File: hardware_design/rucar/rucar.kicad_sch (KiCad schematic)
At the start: 6 parts

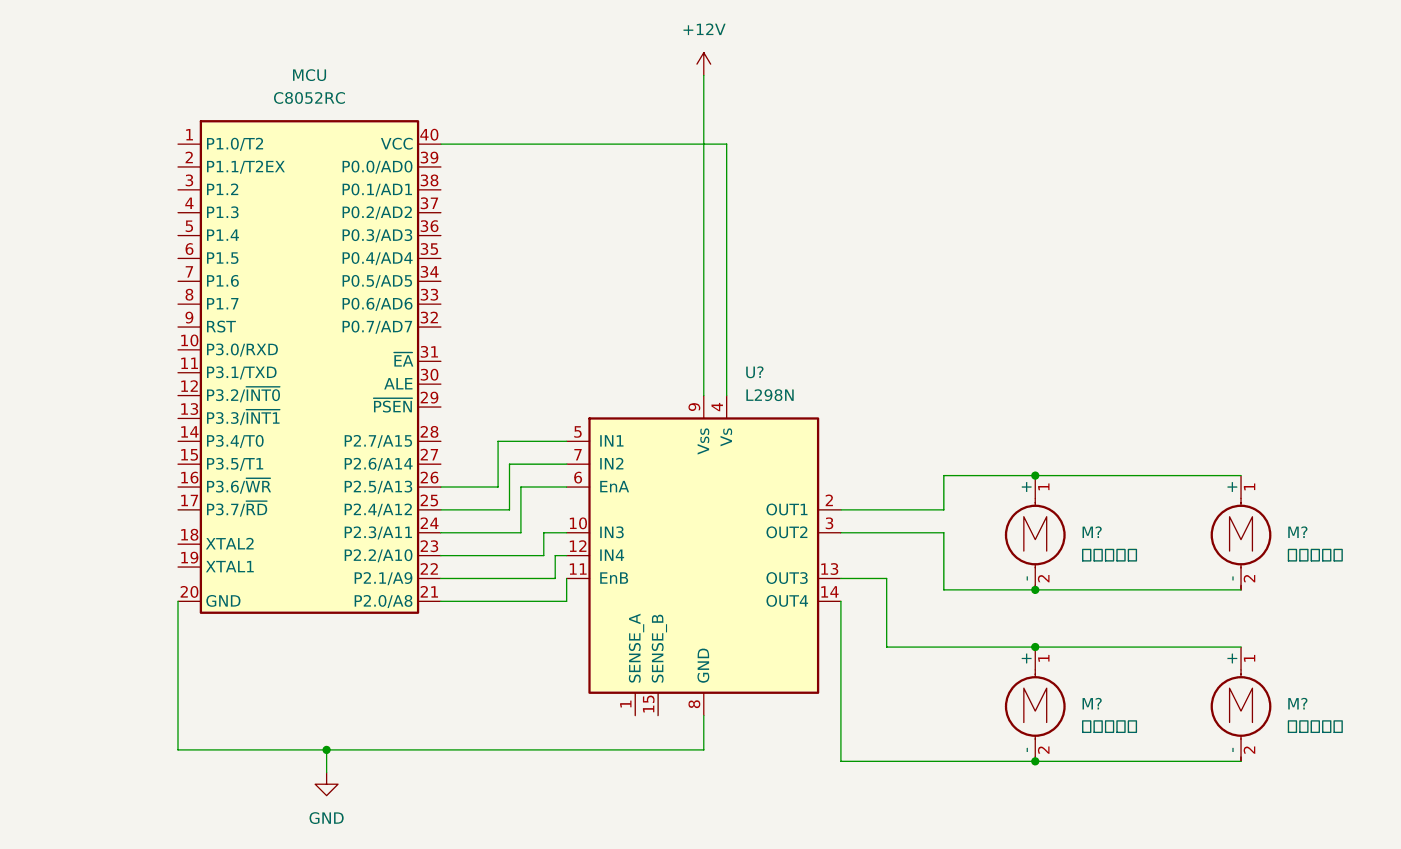
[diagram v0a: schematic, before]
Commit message: finish hardware design.
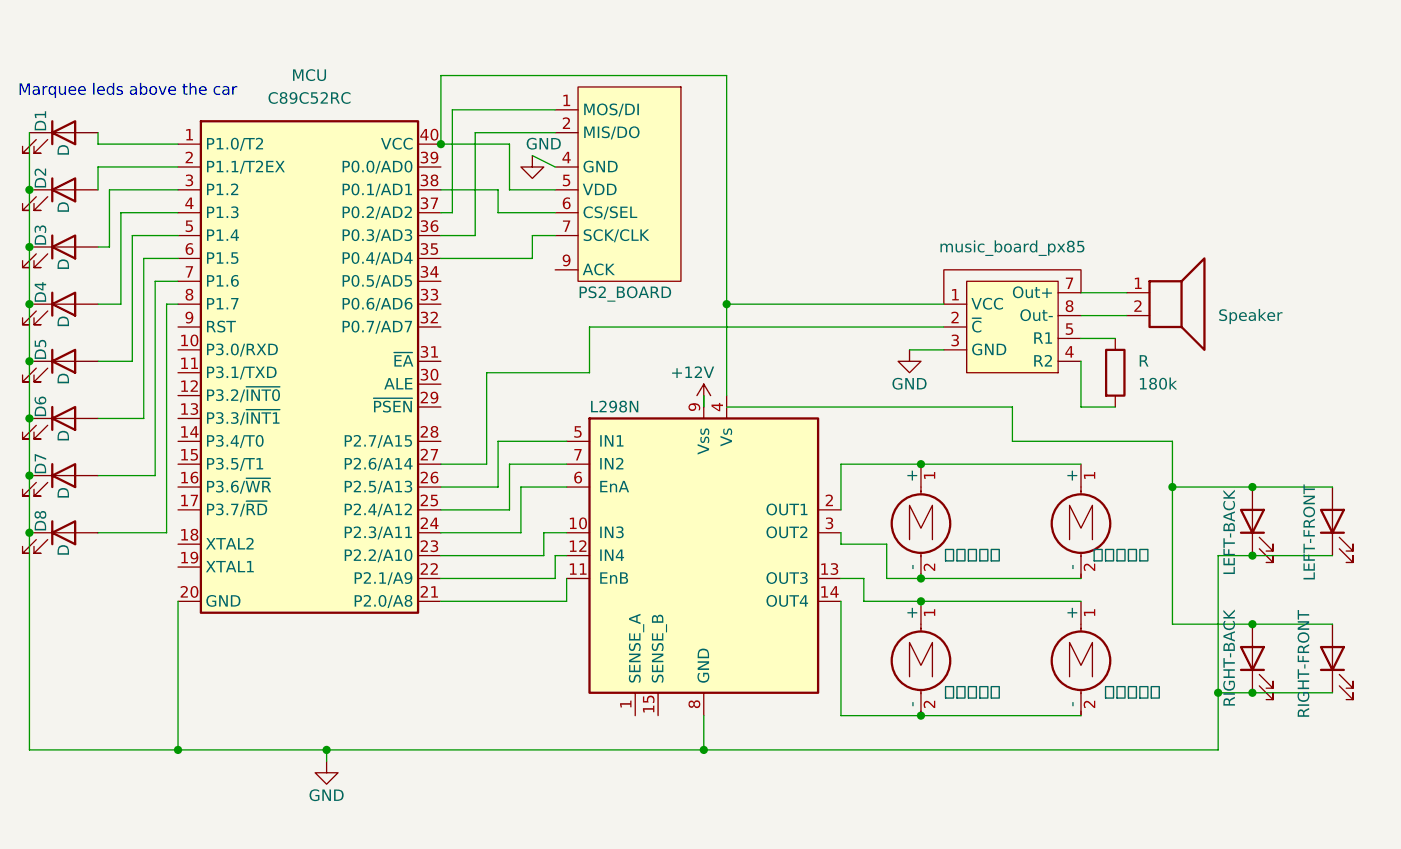
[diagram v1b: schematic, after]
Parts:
- added D: D4, symbol Device:LED
- added D: RIGHT-FRONT, symbol Device:LED
- added D: D8, symbol Device:LED
- added D: D3, symbol Device:LED
- added D: LEFT-FRONT, symbol Device:LED
- added D: LEFT-BACK, symbol Device:LED
- added D: D7, symbol Device:LED
- added D: D1, symbol Device:LED
- added D: D2, symbol Device:LED
- added D: D5, symbol Device:LED
- added D: RIGHT-BACK, symbol Device:LED
- added D: D6, symbol Device:LED
- added LS?: Speaker, symbol Device:Speaker
- added R: 180k, symbol Device:R
- added U?: music_board_px85, symbol Audio:music_board_px85
- added U?: PS2_BOARD, symbol Device:PS2_BOARD
- MCU: value C8052RC -> C89C52RC
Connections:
- net GND: now also D.1 (K), D.1 (K), D.1 (K), D.1 (K), D.1 (K), D.1 (K), D.1 (K), D.1 (K), D.1 (K), D.1 (K), D.1 (K), D.1 (K), U?.3 (GND), U?.4 (GND)
- net at MCU.1 (P1.0/T2): now also D.2 (A)
- net at MCU.2 (P1.1/T2EX): now also D.2 (A)
- net at MCU.27 (P2.6/A14): now also U?.2 (~{C})
- net at MCU.3 (P1.2): now also D.2 (A)
- net at MCU.35 (P0.4/AD4): now also U?.7 (SCK/CLK)
- net at MCU.36 (P0.3/AD3): now also U?.2 (MIS/DO)
- net at MCU.37 (P0.2/AD2): now also U?.1 (MOS/DI)
- net at MCU.38 (P0.1/AD1): now also U?.6 (CS/SEL)
- net at MCU.4 (P1.3): now also D.2 (A)
- net at MCU.40 (VCC), U?.4 (Vs): now also U?.1 (VCC), U?.5 (VDD)
- net at MCU.5 (P1.4): now also D.2 (A)
- net at MCU.6 (P1.5): now also D.2 (A)
- net at MCU.7 (P1.6): now also D.2 (A)
- net at MCU.8 (P1.7): now also D.2 (A)
- new net: R.2, U?.4 (R2)
- new net: R.1, U?.5 (R1)
- new net: LS?.1, U?.7 (Out+)
- new net: LS?.2, U?.8 (Out-)
- new net: D.2 (A), D.2 (A), D.2 (A), D.2 (A)
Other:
- note added: "Marquee leds above the car"
